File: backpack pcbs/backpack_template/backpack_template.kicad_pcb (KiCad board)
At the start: 2 copper layers, 30 x 22.5 mm, 9 parts, among them J1 Conn_01x05_Male, J2 Conn_01x08_Female, J3 Conn_01x08_Female

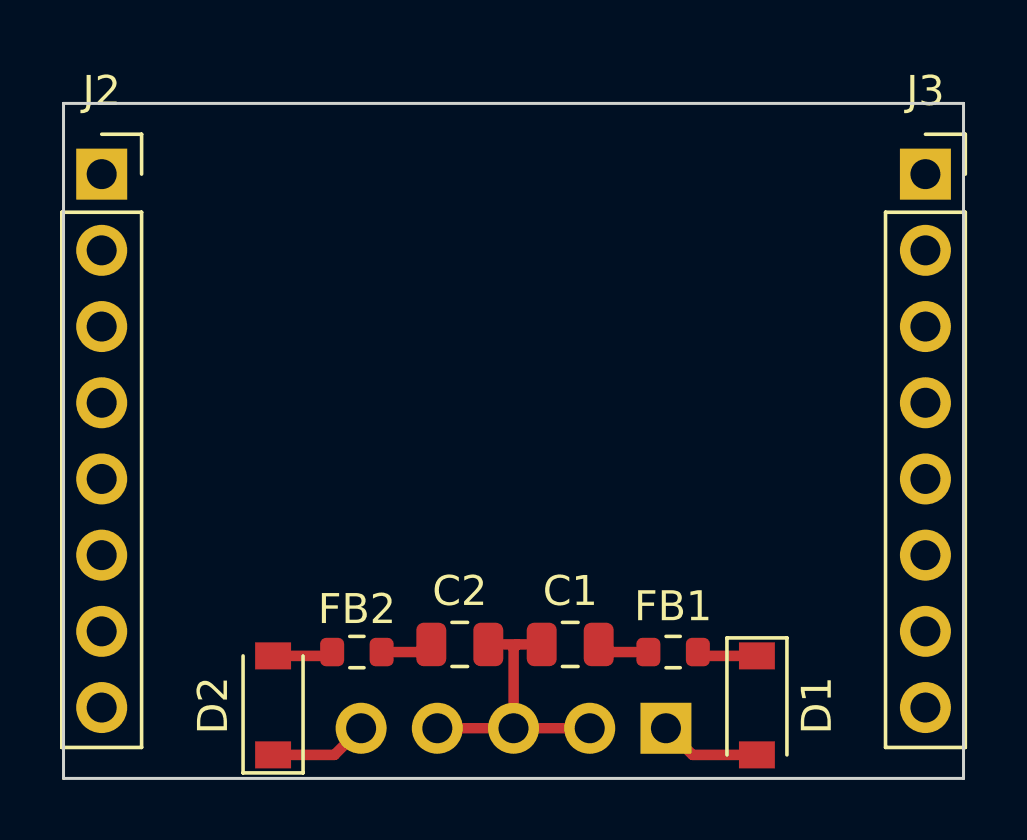
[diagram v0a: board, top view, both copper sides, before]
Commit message: KiCad Save
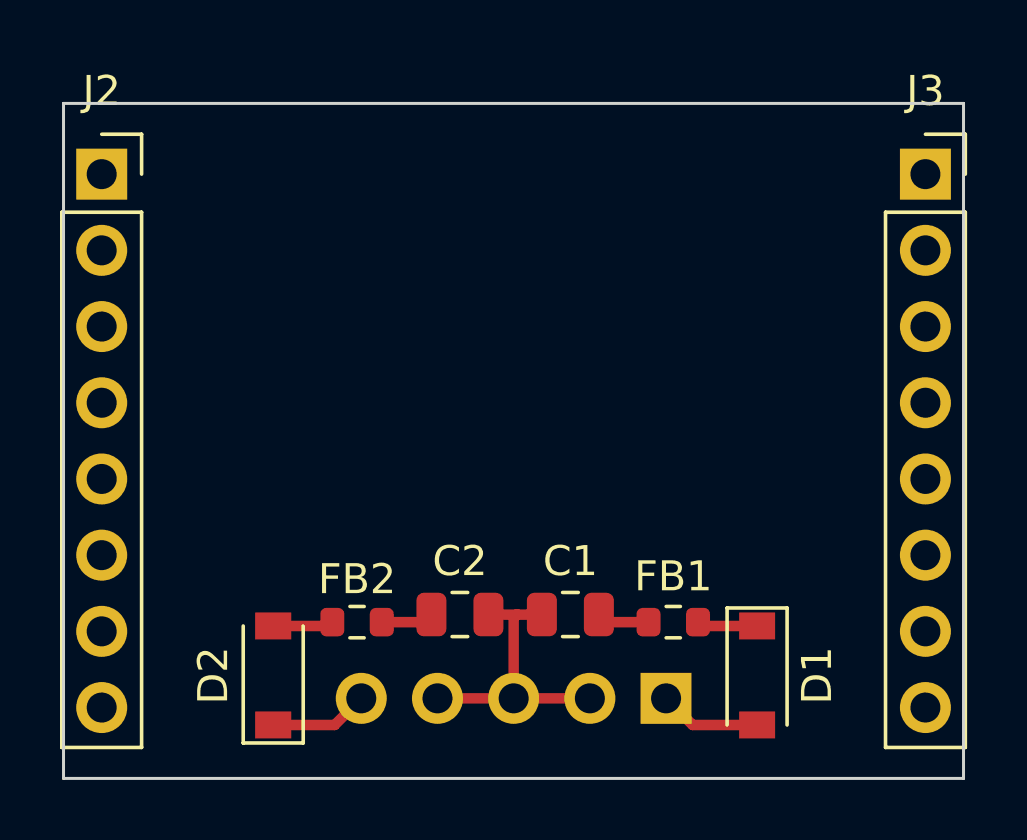
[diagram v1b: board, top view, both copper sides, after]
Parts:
- moved C1 1.00 mm to (16.9, 17.0)
- moved C2 1.00 mm to (13.2, 17.0)
- moved D1 1.00 mm to (23.1, 19.1)
- moved D2 1.00 mm to (6.99, 19.1)
- moved FB1 1.00 mm to (20.3, 17.3)
- moved FB2 1.00 mm to (9.78, 17.3)
- moved J1 1.00 mm to (20.1, 19.8)
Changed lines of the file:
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@@
   (net 23 "unconnected-(J3-Pad8)")
   (footprint "Resistor_SMD:R_0603_1608Metric" (layer "F.Cu")
-    (at 20.32 18.288 180)
+    (at 20.325 17.291 180)
     (descr "Resistor SMD 0603 (1608 Metric), square (rectangular) end terminal, IPC_7351 nominal, (Body size source: IPC-SM-782 page 72, https://www.pcb-3d.com/wordpress/wp-content/uploads/ipc-sm-782a_amendment_1_and_2.pdf), generated with kicad-footprint-generator")
     (tags "resistor")
@@
   )
   (footprint "Diode_SMD:D_SOD-123" (layer "F.Cu")
-    (at 6.985 20.066 90)
+    (at 6.99 19.069 90)
     (descr "SOD-123")
     (tags "SOD-123")
@@
   )
   (footprint "Capacitor_SMD:C_0805_2012Metric" (layer "F.Cu")
-    (at 16.891 18.034 180)
+    (at 16.896 17.037 180)
     (descr "Capacitor SMD 0805 (2012 Metric), square (rectangular) end terminal, IPC_7351 nominal, (Body size source: IPC-SM-782 page 76, https://www.pcb-3d.com/wordpress/wp-content/uploads/ipc-sm-782a_amendment_1_and_2.pdf, https://docs.google.com/spreadsheets/d/1BsfQQcO9C6DZCsRaXUlFlo91Tg2WpOkGARC1WS5S8t0/edit?usp=sharing), generated with kicad-footprint-generator")
     (tags "capacitor")
@@
   )
   (footprint "Resistor_SMD:R_0603_1608Metric" (layer "F.Cu")
-    (at 9.779 18.288)
+    (at 9.784 17.291)
     (descr "Resistor SMD 0603 (1608 Metric), square (rectangular) end terminal, IPC_7351 nominal, (Body size source: IPC-SM-782 page 72, https://www.pcb-3d.com/wordpress/wp-content/uploads/ipc-sm-782a_amendment_1_and_2.pdf), generated with kicad-footprint-generator")
     (tags "resistor")
@@
   )
   (footprint "Diode_SMD:D_SOD-123" (layer "F.Cu")
-    (at 23.114 20.066 -90)
+    (at 23.119 19.069 -90)
     (descr "SOD-123")
     (tags "SOD-123")
@@
   )
   (footprint "Capacitor_SMD:C_0805_2012Metric" (layer "F.Cu")
-    (at 13.208 18.034 180)
+    (at 13.213 17.037 180)
     (descr "Capacitor SMD 0805 (2012 Metric), square (rectangular) end terminal, IPC_7351 nominal, (Body size source: IPC-SM-782 page 76, https://www.pcb-3d.com/wordpress/wp-content/uploads/ipc-sm-782a_amendment_1_and_2.pdf, https://docs.google.com/spreadsheets/d/1BsfQQcO9C6DZCsRaXUlFlo91Tg2WpOkGARC1WS5S8t0/edit?usp=sharing), generated with kicad-footprint-generator")
     (tags "capacitor")
@@
   )
   (footprint "Connector_PinHeader_2.54mm:PinHeader_1x05_P2.54mm_Vertical" (layer "B.Cu")
-    (at 20.08 20.828 90)
+    (at 20.085 19.831 90)
     (descr "Through hole straight pin header, 1x05, 2.54mm pitch, single row")
     (tags "Through hole pin header THT 1x05 2.54mm single row")
@@
   )
   (target plus (at 0 0) (size 5) (width 0.1) (layer "Edge.Cuts"))
-  (segment (start 19.495 18.288) (end 18.095 18.288) (width 0.35) (layer "F.Cu") (net 1))
-  (segment (start 18.095 18.288) (end 17.841 18.034) (width 0.35) (layer "F.Cu") (net 1))
-  (segment (start 15 20.828) (end 15 18.147) (width 0.35) (layer "F.Cu") (net 2))
-  (segment (start 15 18.147) (end 15.113 18.034) (width 0.35) (layer "F.Cu") (net 2))
-  (segment (start 12.46 20.828) (end 17.54 20.828) (width 0.35) (layer "F.Cu") (net 2))
-  (segment (start 14.158 18.034) (end 15.113 18.034) (width 0.35) (layer "F.Cu") (net 2))
-  (segment (start 15.113 18.034) (end 15.941 18.034) (width 0.35) (layer "F.Cu") (net 2))
-  (segment (start 12.004 18.288) (end 12.258 18.034) (width 0.35) (layer "F.Cu") (net 3))
-  (segment (start 10.604 18.288) (end 12.004 18.288) (width 0.35) (layer "F.Cu") (net 3))
-  (segment (start 21.273 18.416) (end 21.145 18.288) (width 0.35) (layer "F.Cu") (net 4))
-  (segment (start 23.114 18.416) (end 21.273 18.416) (width 0.35) (layer "F.Cu") (net 4))
-  (segment (start 20.968 21.716) (end 20.08 20.828) (width 0.35) (layer "F.Cu") (net 5))
-  (segment (start 23.114 21.716) (end 20.968 21.716) (width 0.35) (layer "F.Cu") (net 5))
-  (segment (start 6.985 21.716) (end 9.032 21.716) (width 0.35) (layer "F.Cu") (net 6))
-  (segment (start 9.032 21.716) (end 9.92 20.828) (width 0.35) (layer "F.Cu") (net 6))
-  (segment (start 8.826 18.416) (end 8.954 18.288) (width 0.35) (layer "F.Cu") (net 7))
-  (segment (start 6.985 18.416) (end 8.826 18.416) (width 0.35) (layer "F.Cu") (net 7))
+  (segment (start 19.5 17.291) (end 18.1 17.291) (width 0.35) (layer "F.Cu") (net 1))
+  (segment (start 18.1 17.291) (end 17.846 17.037) (width 0.35) (layer "F.Cu") (net 1))
+  (segment (start 15.005 19.831) (end 15.005 17.15) (width 0.35) (layer "F.Cu") (net 2))
+  (segment (start 15.005 17.15) (end 15.118 17.037) (width 0.35) (layer "F.Cu") (net 2))
+  (segment (start 12.465 19.831) (end 17.545 19.831) (width 0.35) (layer "F.Cu") (net 2))
+  (segment (start 14.163 17.037) (end 15.118 17.037) (width 0.35) (layer "F.Cu") (net 2))
+  (segment (start 15.118 17.037) (end 15.946 17.037) (width 0.35) (layer "F.Cu") (net 2))
+  (segment (start 12.009 17.291) (end 12.263 17.037) (width 0.35) (layer "F.Cu") (net 3))
+  (segment (start 10.609 17.291) (end 12.009 17.291) (width 0.35) (layer "F.Cu") (net 3))
+  (segment (start 21.278 17.419) (end 21.15 17.291) (width 0.35) (layer "F.Cu") (net 4))
+  (segment (start 23.119 17.419) (end 21.278 17.419) (width 0.35) (layer "F.Cu") (net 4))
+  (segment (start 20.973 20.719) (end 20.085 19.831) (width 0.35) (layer "F.Cu") (net 5))
+  (segment (start 23.119 20.719) (end 20.973 20.719) (width 0.35) (layer "F.Cu") (net 5))
+  (segment (start 6.99 20.719) (end 9.037 20.719) (width 0.35) (layer "F.Cu") (net 6))
+  (segment (start 9.037 20.719) (end 9.925 19.831) (width 0.35) (layer "F.Cu") (net 6))
+  (segment (start 8.831 17.419) (end 8.959 17.291) (width 0.35) (layer "F.Cu") (net 7))
+  (segment (start 6.99 17.419) (end 8.831 17.419) (width 0.35) (layer "F.Cu") (net 7))
   (zone (net 0) (net_name "") (layer "B.SilkS") (hatch none 0.508)
     (connect_pads (clearance 0.508))
